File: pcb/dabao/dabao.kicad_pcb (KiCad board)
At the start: 2 copper layers, 127.4 x 106.6 mm, 74 parts, among them J1 Conn_01x05, J2 USB_C_Receptacle_USB2.0_16P, J3 Conn_01x04, J4 MagConn_01x04_Pin, J5 Conn_Battery, J7 Conn_01x04, J8 Display, SW1 SW_RESET, SW2 SW_POWER, U1 nice_nano, U2 MCP23017_SP

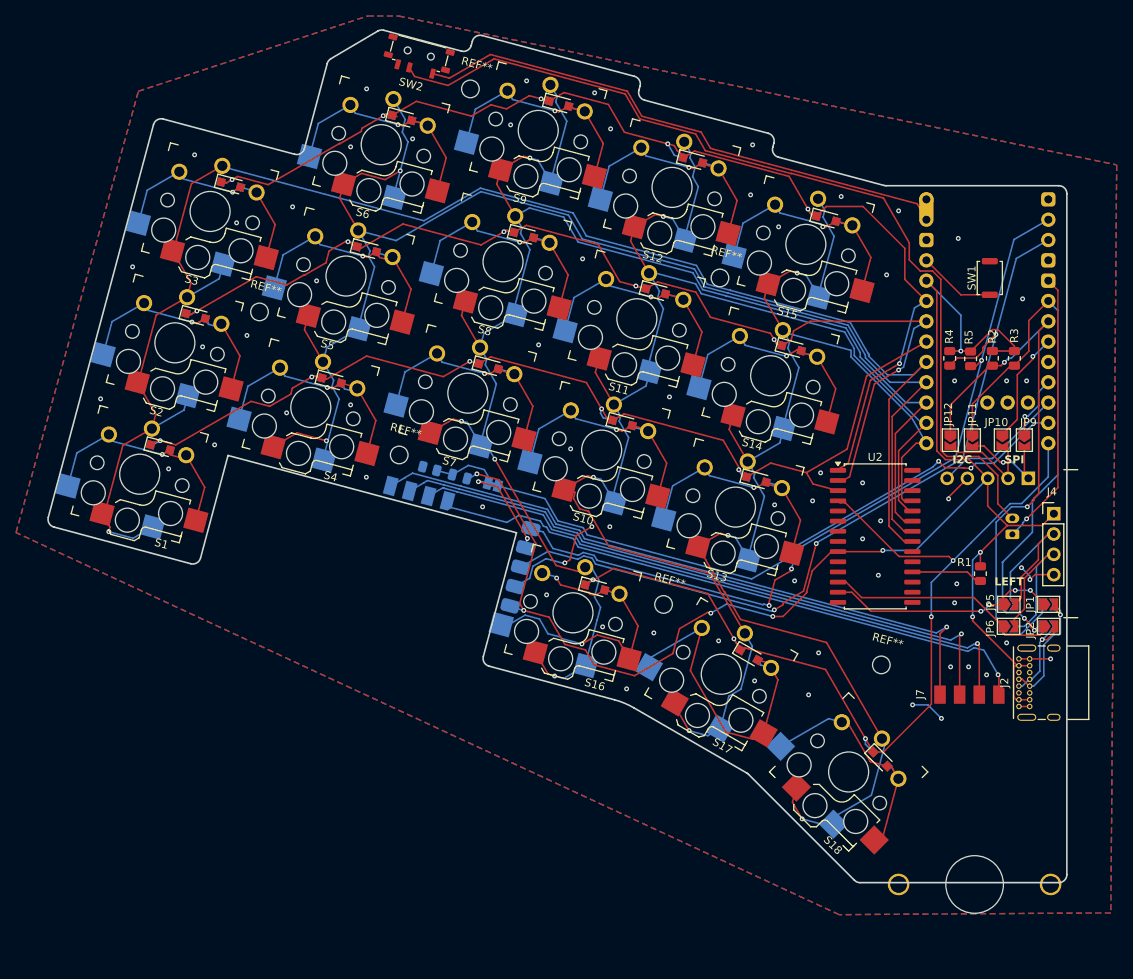
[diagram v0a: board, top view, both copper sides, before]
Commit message: Update pcb outline, final-ish drc checks
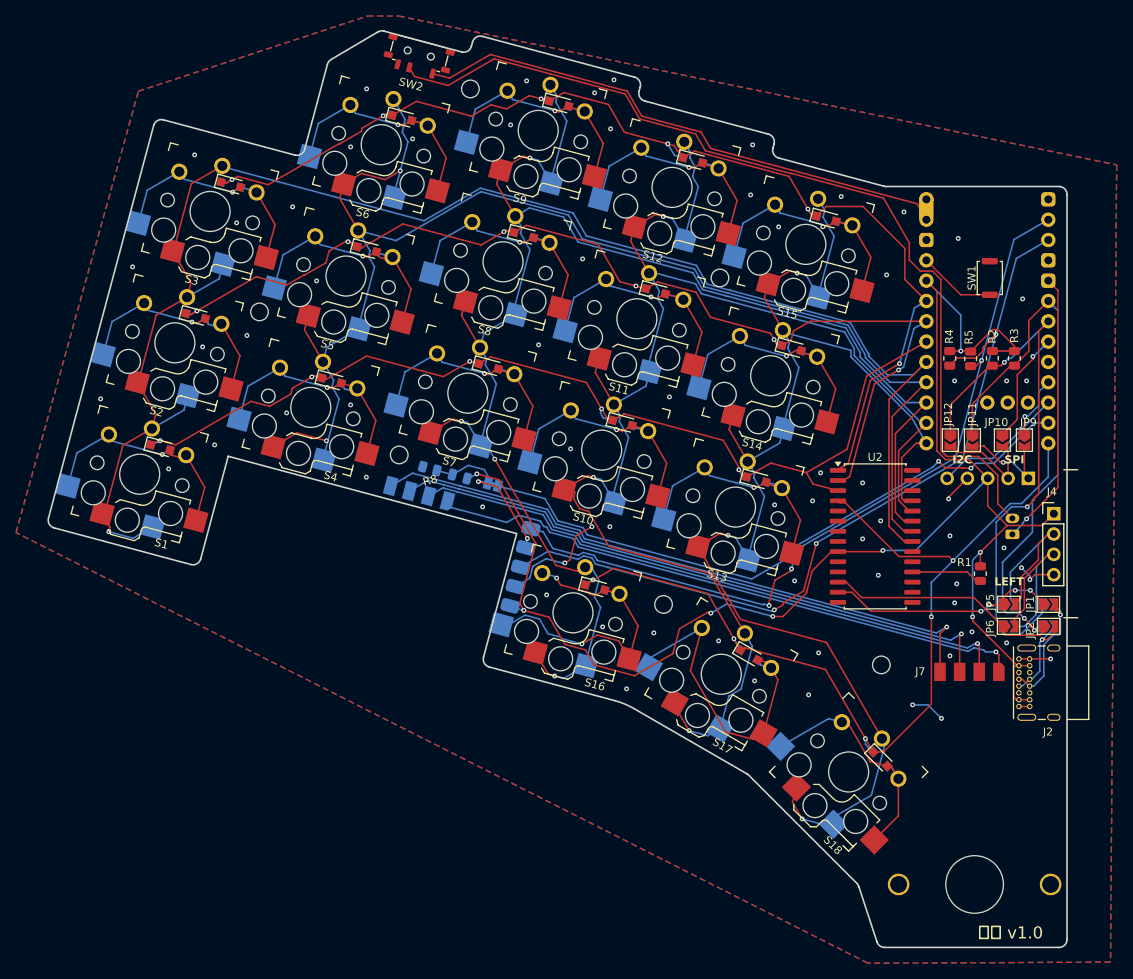
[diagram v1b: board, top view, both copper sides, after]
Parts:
- moved J7 2.84 mm to (201.2, 133.5)
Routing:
- net Net-(J3-Pin_4): track 82.8 -> 80.0 mm
- net Net-(J3-Pin_2): track 79.4 -> 76.6 mm
- net Net-(J3-Pin_3): track 81.1 -> 78.6 mm
- net Net-(J3-Pin_1): track 77.5 -> 75.7 mm
- net /row_top: track 141.8 -> 141.2 mm
- net GND: vias 68 -> 70
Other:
- board size 127.4 x 106.6 mm -> 127.4 x 114.6 mm
- board text added: "打包 v1.0"
